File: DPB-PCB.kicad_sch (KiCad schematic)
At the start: 6 parts, among them U1 ESP32-S3-WROOM-1-N4R2

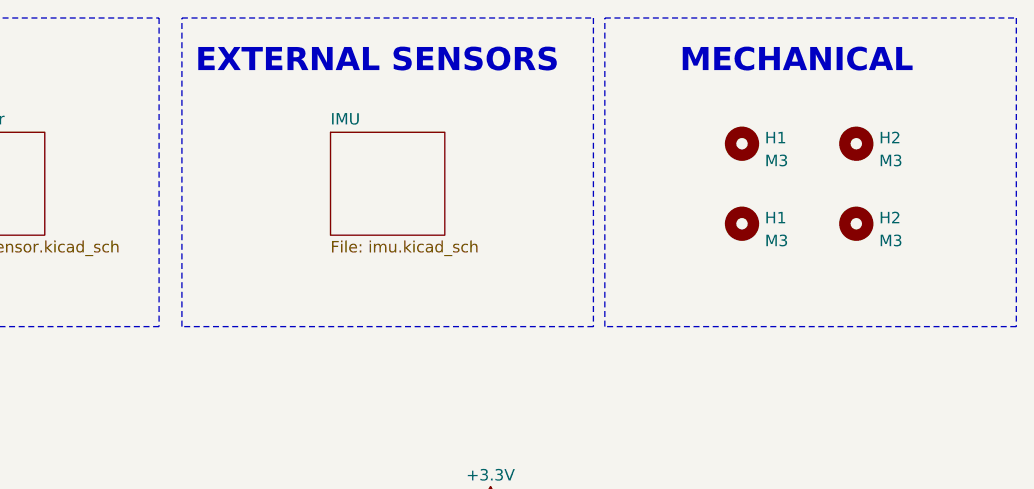
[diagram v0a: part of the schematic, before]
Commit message: Divided project
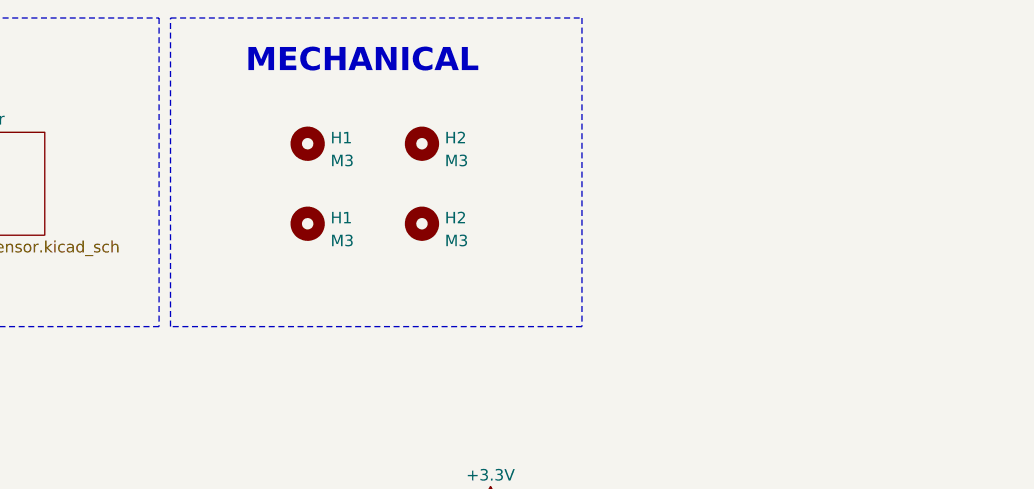
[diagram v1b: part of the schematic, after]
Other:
- removed sheet IMU
- note removed: "EXTERNAL SENSORS"
- moved on the sheet: H1, H2
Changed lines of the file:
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@@
     (stroke (width 0) (type default))
   )
-  (rectangle (start 138.43 13.97) (end 184.15 48.26)
-    (stroke (width 0) (type dash))
-    (fill (type none))
-  )
-  (rectangle (start 185.42 13.97) (end 231.14 48.26)
+  (rectangle (start 137.16 13.97) (end 182.88 48.26)
     (stroke (width 0) (type dash))
     (fill (type none))
@@
     (fill (type none))
   )
-  (text "EXTERNAL SENSORS" (at 180.34 20.32 0)
-    (effects (font (size 2.5654 2.5654) (thickness 0.5131) bold) (justify right bottom))
-  )
-  (text "MECHANICAL" (at 219.71 20.32 0)
+  (text "MECHANICAL" (at 171.45 20.32 0)
     (effects (font (size 2.5654 2.5654) (thickness 0.5131) bold) (justify right bottom))
   )
@@
     )
   )
-  (symbol (lib_id "Mechanical:MountingHole") (at 213.36 27.94 0) (unit 1)
-    (in_bom yes) (on_board yes) (dnp no) (fields_autoplaced)
-    (property "Reference" "H2" (at 215.9 27.305 0)
-      (effects (font (size 1.27 1.27)) (justify left))
-    )
-    (property "Value" "M3" (at 215.9 29.845 0)
-      (effects (font (size 1.27 1.27)) (justify left))
-    )
-    (property "Footprint" "MountingHole:MountingHole_3.2mm_M3_Pad_TopBottom" (at 213.36 27.94 0)
-      (effects (font (size 1.27 1.27)) hide)
-    )
-    (property "Datasheet" "~" (at 213.36 27.94 0)
-      (effects (font (size 1.27 1.27)) hide)
-    )
-    (instances
-      (project "DPB-PCB"
-        (path "/0a09ce58-c923-4e96-b56b-0b86aca559ed/5d947656-d224-44e7-8ee3-5b0d738fb419"
-          (reference "H2") (unit 1)
-        )
+  (symbol (lib_id "Mechanical:MountingHole") (at 165.1 27.94 0) (unit 1)
+    (in_bom yes) (on_board yes) (dnp no) (fields_autoplaced)
+    (property "Reference" "H2" (at 167.64 27.305 0)
+      (effects (font (size 1.27 1.27)) (justify left))
+    )
+    (property "Value" "M3" (at 167.64 29.845 0)
+      (effects (font (size 1.27 1.27)) (justify left))
+    )
+    (property "Footprint" "MountingHole:MountingHole_3.2mm_M3_Pad_TopBottom" (at 165.1 27.94 0)
+      (effects (font (size 1.27 1.27)) hide)
+    )
+    (property "Datasheet" "~" (at 165.1 27.94 0)
+      (effects (font (size 1.27 1.27)) hide)
+    )
+    (instances
+      (project "DPB-PCB"
         (path "/0a09ce58-c923-4e96-b56b-0b86aca559ed"
           (reference "H4") (unit 1)
@@
     )
   )
-  (symbol (lib_id "Mechanical:MountingHole") (at 200.66 36.83 0) (unit 1)
-    (in_bom yes) (on_board yes) (dnp no) (fields_autoplaced)
-    (property "Reference" "H1" (at 203.2 36.195 0)
-      (effects (font (size 1.27 1.27)) (justify left))
-    )
-    (property "Value" "M3" (at 203.2 38.735 0)
-      (effects (font (size 1.27 1.27)) (justify left))
-    )
-    (property "Footprint" "MountingHole:MountingHole_3.2mm_M3_Pad_TopBottom" (at 200.66 36.83 0)
-      (effects (font (size 1.27 1.27)) hide)
-    )
-    (property "Datasheet" "~" (at 200.66 36.83 0)
-      (effects (font (size 1.27 1.27)) hide)
-    )
-    (instances
-      (project "DPB-PCB"
-        (path "/0a09ce58-c923-4e96-b56b-0b86aca559ed/5d947656-d224-44e7-8ee3-5b0d738fb419"
-          (reference "H1") (unit 1)
-        )
+  (symbol (lib_id "Mechanical:MountingHole") (at 152.4 36.83 0) (unit 1)
+    (in_bom yes) (on_board yes) (dnp no) (fields_autoplaced)
+    (property "Reference" "H1" (at 154.94 36.195 0)
+      (effects (font (size 1.27 1.27)) (justify left))
+    )
+    (property "Value" "M3" (at 154.94 38.735 0)
+      (effects (font (size 1.27 1.27)) (justify left))
+    )
+    (property "Footprint" "MountingHole:MountingHole_3.2mm_M3_Pad_TopBottom" (at 152.4 36.83 0)
+      (effects (font (size 1.27 1.27)) hide)
+    )
+    (property "Datasheet" "~" (at 152.4 36.83 0)
+      (effects (font (size 1.27 1.27)) hide)
+    )
+    (instances
+      (project "DPB-PCB"
         (path "/0a09ce58-c923-4e96-b56b-0b86aca559ed"
           (reference "H5") (unit 1)
@@
     )
   )
-  (symbol (lib_id "Mechanical:MountingHole") (at 213.36 36.83 0) (unit 1)
-    (in_bom yes) (on_board yes) (dnp no) (fields_autoplaced)
-    (property "Reference" "H2" (at 215.9 36.195 0)
-      (effects (font (size 1.27 1.27)) (justify left))
-    )
-    (property "Value" "M3" (at 215.9 38.735 0)
-      (effects (font (size 1.27 1.27)) (justify left))
-    )
-    (property "Footprint" "MountingHole:MountingHole_3.2mm_M3_Pad_TopBottom" (at 213.36 36.83 0)
-      (effects (font (size 1.27 1.27)) hide)
-    )
-    (property "Datasheet" "~" (at 213.36 36.83 0)
-      (effects (font (size 1.27 1.27)) hide)
-    )
-    (instances
-      (project "DPB-PCB"
-        (path "/0a09ce58-c923-4e96-b56b-0b86aca559ed/5d947656-d224-44e7-8ee3-5b0d738fb419"
-          (reference "H2") (unit 1)
-        )
+  (symbol (lib_id "Mechanical:MountingHole") (at 165.1 36.83 0) (unit 1)
+    (in_bom yes) (on_board yes) (dnp no) (fields_autoplaced)
+    (property "Reference" "H2" (at 167.64 36.195 0)
+      (effects (font (size 1.27 1.27)) (justify left))
+    )
+    (property "Value" "M3" (at 167.64 38.735 0)
+      (effects (font (size 1.27 1.27)) (justify left))
+    )
+    (property "Footprint" "MountingHole:MountingHole_3.2mm_M3_Pad_TopBottom" (at 165.1 36.83 0)
+      (effects (font (size 1.27 1.27)) hide)
+    )
+    (property "Datasheet" "~" (at 165.1 36.83 0)
+      (effects (font (size 1.27 1.27)) hide)
+    )
+    (instances
+      (project "DPB-PCB"
         (path "/0a09ce58-c923-4e96-b56b-0b86aca559ed"
           (reference "H6") (unit 1)
@@
     )
   )
-  (symbol (lib_id "Mechanical:MountingHole") (at 200.66 27.94 0) (unit 1)
-    (in_bom yes) (on_board yes) (dnp no) (fields_autoplaced)
-    (property "Reference" "H1" (at 203.2 27.305 0)
-      (effects (font (size 1.27 1.27)) (justify left))
-    )
-    (property "Value" "M3" (at 203.2 29.845 0)
-      (effects (font (size 1.27 1.27)) (justify left))
-    )
-    (property "Footprint" "MountingHole:MountingHole_3.2mm_M3_Pad_TopBottom" (at 200.66 27.94 0)
-      (effects (font (size 1.27 1.27)) hide)
-    )
-    (property "Datasheet" "~" (at 200.66 27.94 0)
-      (effects (font (size 1.27 1.27)) hide)
-    )
-    (instances
-      (project "DPB-PCB"
-        (path "/0a09ce58-c923-4e96-b56b-0b86aca559ed/5d947656-d224-44e7-8ee3-5b0d738fb419"
-          (reference "H1") (unit 1)
-        )
+  (symbol (lib_id "Mechanical:MountingHole") (at 152.4 27.94 0) (unit 1)
+    (in_bom yes) (on_board yes) (dnp no) (fields_autoplaced)
+    (property "Reference" "H1" (at 154.94 27.305 0)
+      (effects (font (size 1.27 1.27)) (justify left))
+    )
+    (property "Value" "M3" (at 154.94 29.845 0)
+      (effects (font (size 1.27 1.27)) (justify left))
+    )
+    (property "Footprint" "MountingHole:MountingHole_3.2mm_M3_Pad_TopBottom" (at 152.4 27.94 0)
+      (effects (font (size 1.27 1.27)) hide)
+    )
+    (property "Datasheet" "~" (at 152.4 27.94 0)
+      (effects (font (size 1.27 1.27)) hide)
+    )
+    (instances
+      (project "DPB-PCB"
         (path "/0a09ce58-c923-4e96-b56b-0b86aca559ed"
           (reference "H3") (unit 1)
@@
       )
     )
-  )
-  (sheet (at 154.94 26.67) (size 12.7 11.43) (fields_autoplaced)
-    (stroke (width 0.1524) (type solid))
-    (fill (color 0 0 0 0.0000))
-    (property "Sheetname" "IMU" (at 154.94 25.9584 0)
-      (effects (font (size 1.27 1.27)) (justify left bottom))
-    )
-    (property "Sheetfile" "imu.kicad_sch" (at 154.94 38.6846 0)
-      (effects (font (size 1.27 1.27)) (justify left top))
-    )
-    (instances
-      (project "DPB-PCB"
-        (path "/0a09ce58-c923-4e96-b56b-0b86aca559ed" (page "5"))
-      )
-    )

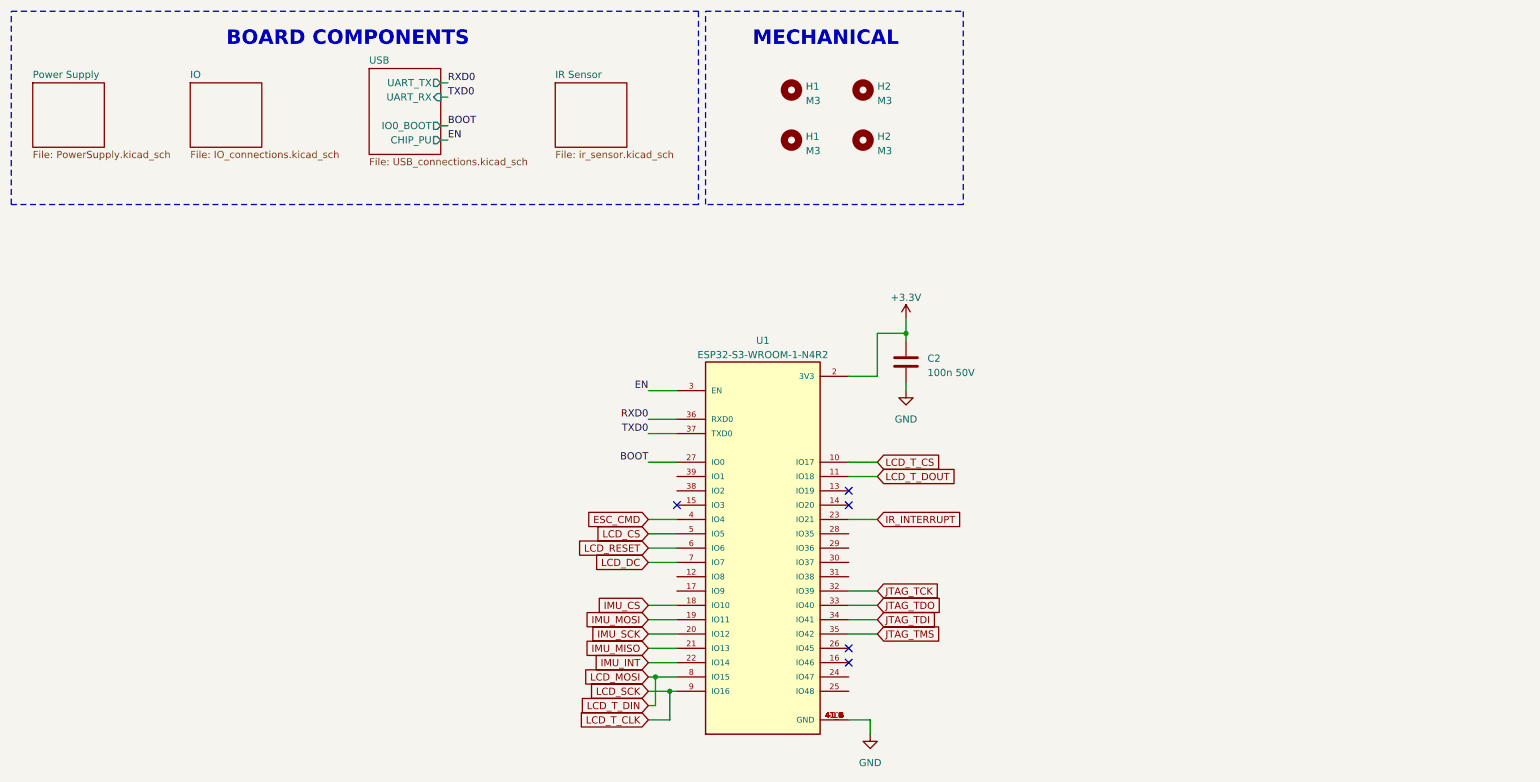
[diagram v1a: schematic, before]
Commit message: DPB mainboard_v1 completed
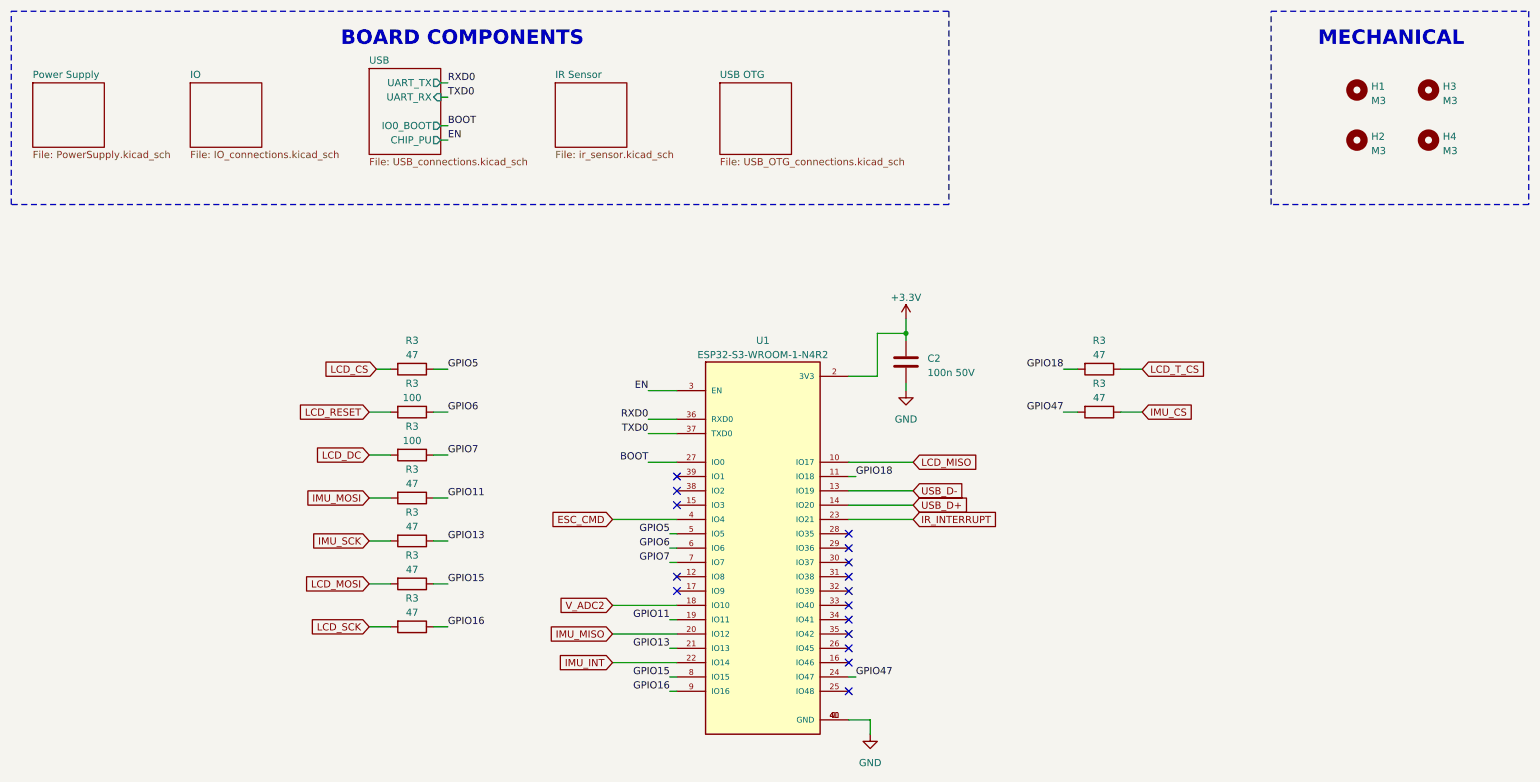
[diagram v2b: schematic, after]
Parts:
- added R3 (x7): 47, Resistor_SMD:R_0402_1005Metric, symbol Device:R
- added R3 (x2): 100, Resistor_SMD:R_0402_1005Metric, symbol Device:R
- renumbered H1 to H2, H2 to H3, H2 to H4
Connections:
- net GND: now also U1.41 (GND); no longer U1.41_1 (GND), U1.41_2 (GND), U1.41_3 (GND), U1.41_4 (GND), U1.41_5 (GND), U1.41_6 (GND), U1.41_7 (GND), U1.41_8 (GND), U1.41_9 (GND)
- net IMU_CS: now also R3.1; no longer U1.18 (IO10)
- net IMU_MISO: now also U1.20 (IO12); no longer U1.21 (IO13)
- net IMU_MOSI: now also R3.2; no longer U1.19 (IO11)
- net IMU_SCK: now also R3.2; no longer U1.20 (IO12)
- net LCD_CS: now also R3.2; no longer U1.5 (IO5)
- net LCD_DC: now also R3.2; no longer U1.7 (IO7)
- net LCD_MOSI: now also R3.2; no longer U1.8 (IO15)
- net LCD_RESET: now also R3.2; no longer U1.6 (IO6)
- net LCD_SCK: now also R3.2; no longer U1.9 (IO16)
- net LCD_T_CS: now also R3.1; no longer U1.10 (IO17)
- net USB_D-: now reaches U1.13 (IO19)
- net USB_D+: now reaches U1.14 (IO20)
- net GPIO47: now reaches U1.24 (IO47)
- net GPIO47: now also R3.2
- net JTAG_TCK: no longer names the net of U1.32 (IO39)
- net JTAG_TDI: no longer names the net of U1.34 (IO41)
- net JTAG_TDO: no longer names the net of U1.33 (IO40)
- net JTAG_TMS: no longer names the net of U1.35 (IO42)
- net LCD_T_DOUT renamed GPIO18
- net GPIO18: now also R3.2
- new net GPIO11: R3.1, U1.19 (IO11)
- new net GPIO13: R3.1, U1.21 (IO13)
- new net GPIO15: R3.1, U1.8 (IO15)
- new net GPIO16: R3.1, U1.9 (IO16)
- new net GPIO5: R3.1, U1.5 (IO5)
- new net GPIO6: R3.1, U1.6 (IO6)
- new net GPIO7: R3.1, U1.7 (IO7)
- new net LCD_MISO: U1.10 (IO17)
- new net V_ADC2: U1.18 (IO10)
- no-connect marks 5 -> 16
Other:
- added sheet USB OTG (USB_OTG_connections.kicad_sch)
- moved on the sheet: H1, H2, H3, H4

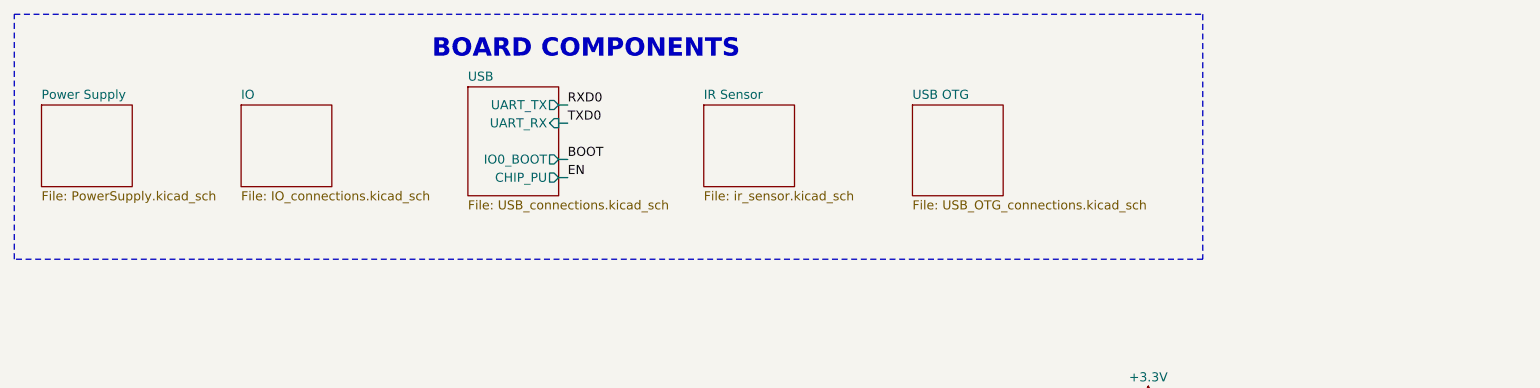
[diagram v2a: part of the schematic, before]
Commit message: On production | V0.1
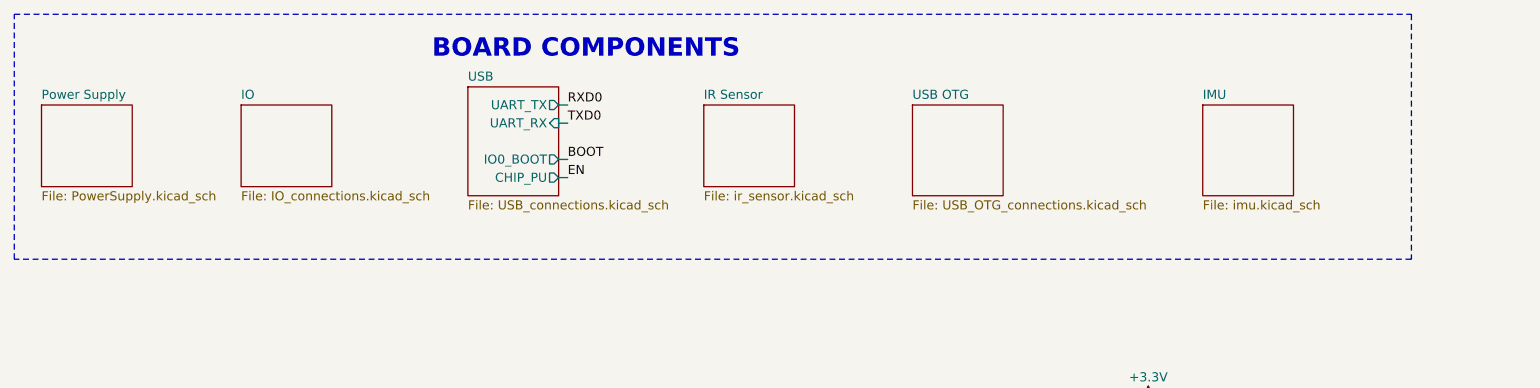
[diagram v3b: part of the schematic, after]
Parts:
- H1, H2, H3, H4: now left out of the parts list
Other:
- added sheet IMU (imu.kicad_sch)
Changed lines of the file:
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@@
     (fill (type none))
   )
-  (rectangle (start 13.97 13.97) (end 180.34 48.26)
+  (rectangle (start 13.97 13.97) (end 209.55 48.26)
     (stroke (width 0) (type dash))
     (fill (type none))
@@
   )
   (symbol (lib_id "Mechanical:MountingHole") (at 265.43 27.94 0) (unit 1)
-    (in_bom yes) (on_board yes) (dnp no) (fields_autoplaced)
+    (in_bom no) (on_board yes) (dnp no) (fields_autoplaced)
     (property "Reference" "H3" (at 267.97 27.305 0)
       (effects (font (size 1.27 1.27)) (justify left))
@@
   )
   (symbol (lib_id "Mechanical:MountingHole") (at 252.73 36.83 0) (unit 1)
-    (in_bom yes) (on_board yes) (dnp no) (fields_autoplaced)
+    (in_bom no) (on_board yes) (dnp no) (fields_autoplaced)
     (property "Reference" "H2" (at 255.27 36.195 0)
       (effects (font (size 1.27 1.27)) (justify left))
@@
   )
   (symbol (lib_id "Mechanical:MountingHole") (at 265.43 36.83 0) (unit 1)
-    (in_bom yes) (on_board yes) (dnp no) (fields_autoplaced)
+    (in_bom no) (on_board yes) (dnp no) (fields_autoplaced)
     (property "Reference" "H4" (at 267.97 36.195 0)
       (effects (font (size 1.27 1.27)) (justify left))
@@
   )
   (symbol (lib_id "Mechanical:MountingHole") (at 252.73 27.94 0) (unit 1)
-    (in_bom yes) (on_board yes) (dnp no) (fields_autoplaced)
+    (in_bom no) (on_board yes) (dnp no) (fields_autoplaced)
     (property "Reference" "H1" (at 255.27 27.305 0)
       (effects (font (size 1.27 1.27)) (justify left))
@@
       )
     )
+  )
+  (sheet (at 180.34 26.67) (size 12.7 12.7) (fields_autoplaced)
+    (stroke (width 0.1524) (type solid))
+    (fill (color 0 0 0 0.0000))
+    (property "Sheetname" "IMU" (at 180.34 25.9584 0)
+      (effects (font (size 1.27 1.27)) (justify left bottom))
+    )
+    (property "Sheetfile" "imu.kicad_sch" (at 180.34 39.9546 0)
+      (effects (font (size 1.27 1.27)) (justify left top))
+    )
+    (instances
+      (project "DPB-PCB"
+        (path "/0a09ce58-c923-4e96-b56b-0b86aca559ed" (page "7"))
+      )
+    )
